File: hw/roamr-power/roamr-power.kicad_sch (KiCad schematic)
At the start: 12 parts, among them J1 Conn_01x02_Socket, J2 Conn_01x02_Socket, J3 Conn_01x02_Socket, P2 USB_C_Plug_USB2.0

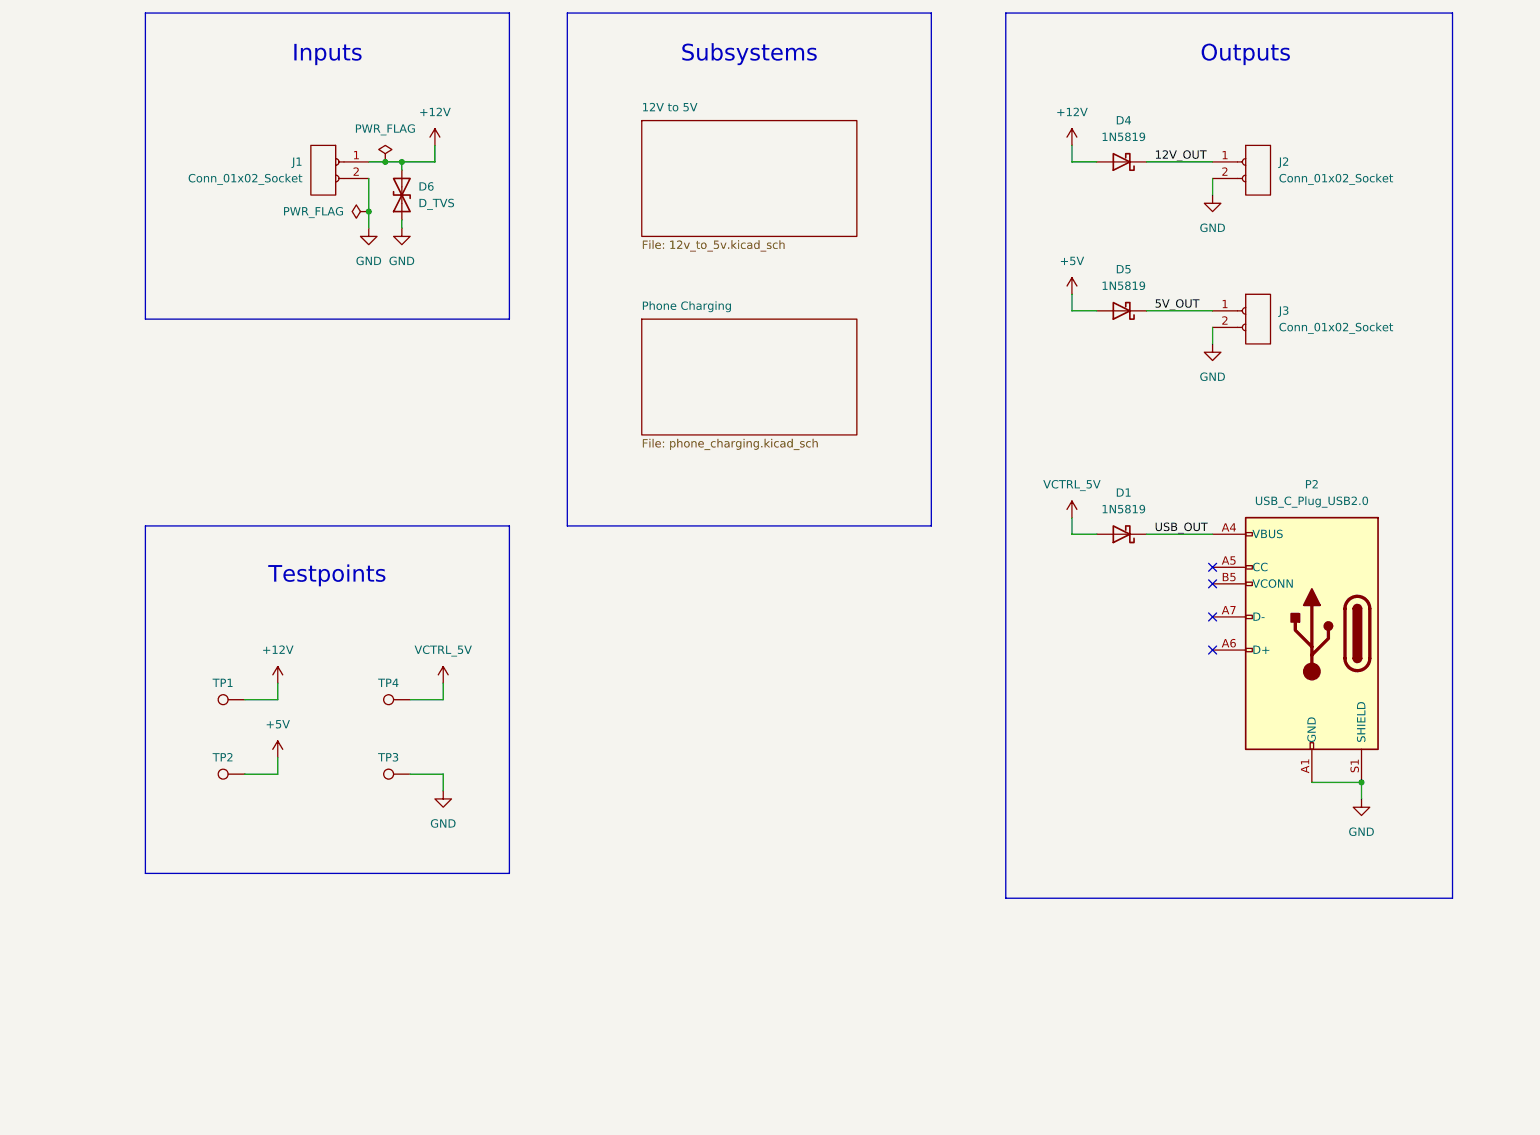
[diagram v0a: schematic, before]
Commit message: pcb schematic and layout updated
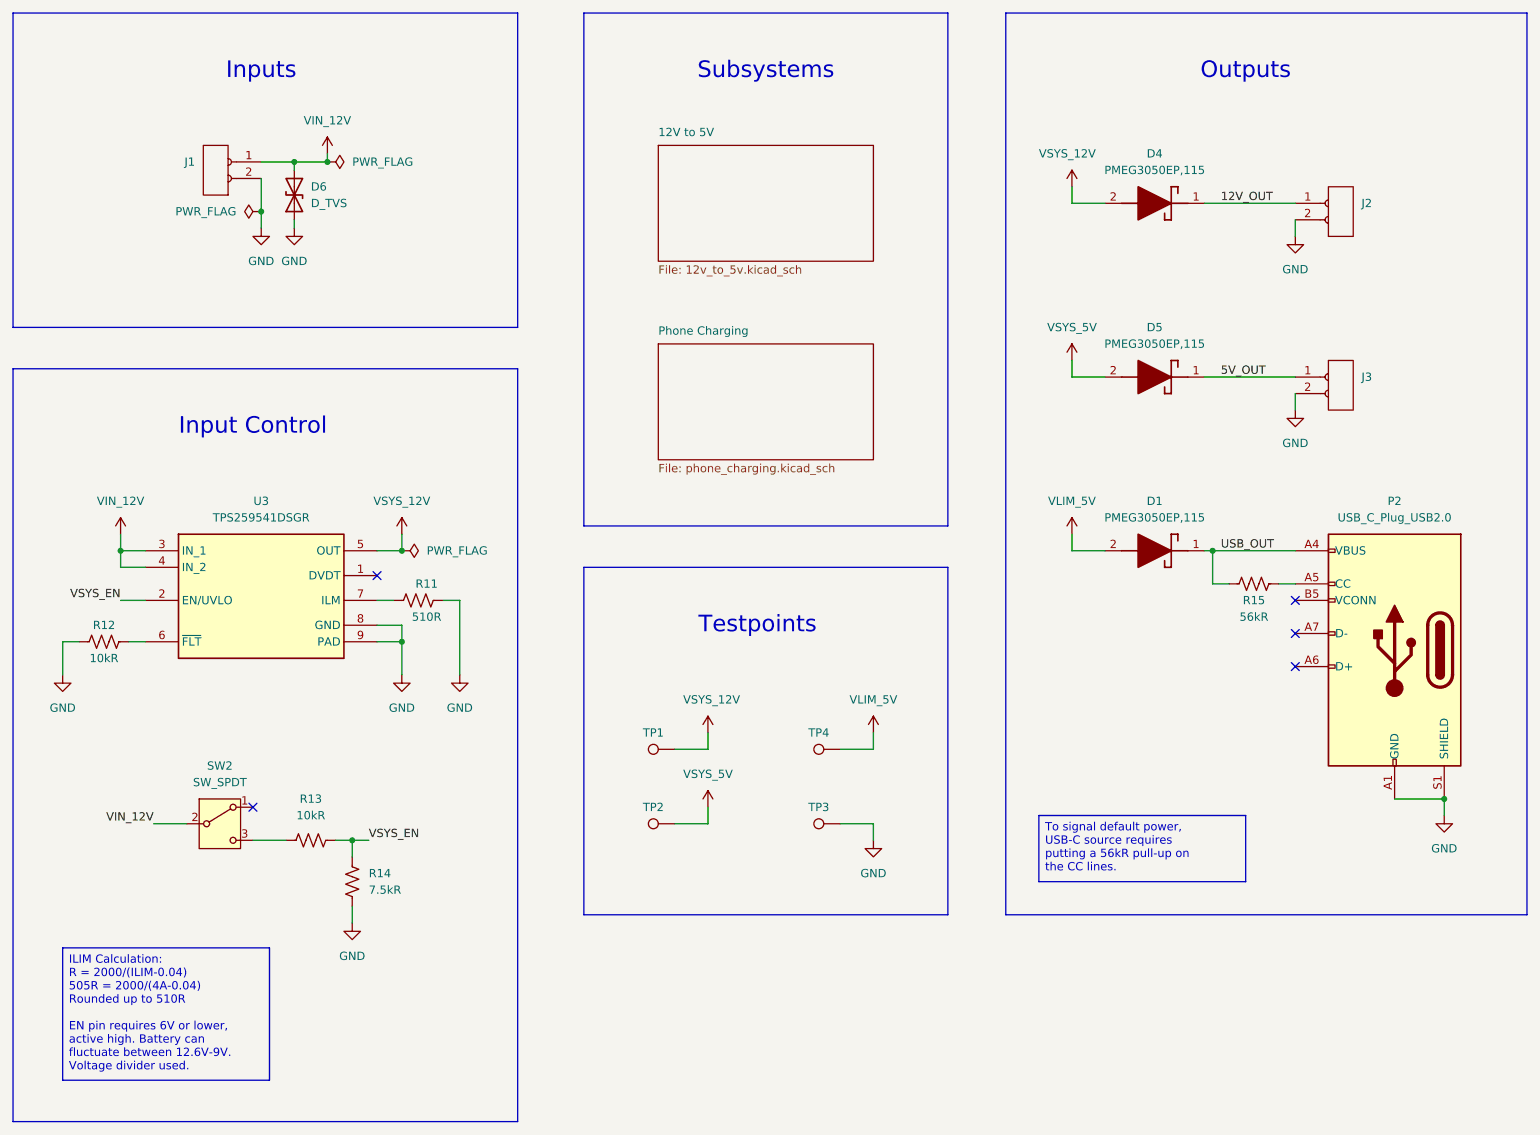
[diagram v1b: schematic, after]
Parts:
- removed D1, D4, D5: 1N5819, Diode_THT:D_DO-41_SOD81_P10.16mm_Horizontal, symbol Diode:1N5819
- added D1, D4, D5: PMEG3050EP,115, PMEG3050EP:PMEG3050EP115, symbol PMEG3050EP_115:PMEG3050EP,115
- added R11: 510R, Resistor_SMD:R_0603_1608Metric, symbol Device:R_US
- added R12, R13: 10kR, Resistor_SMD:R_0603_1608Metric, symbol Device:R_US
- added R14: 7.5kR, Resistor_SMD:R_0603_1608Metric, symbol Device:R_US
- added R15: 56kR, Resistor_SMD:R_0603_1608Metric, symbol Device:R_US
- added SW2: SW_SPDT, OS102011MS2QN1:OS102011MA1QN1, symbol Switch:SW_SPDT
- added U3: TPS259541DSGR, TPS259541DSGR:SON50P200X200X80-9N, symbol TPS259541DSGR:TPS259541DSGR
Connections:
- net 12V_OUT: now also D4.1 (K)
- net 5V_OUT: now also D5.1 (K)
- net GND: now also R11.2, R12.1, R14.2, U3.8 (GND), U3.9 (PAD)
- net USB_OUT: now also D1.1 (K), R15.1
- net at P2.A5 (CC): now also R15.2
- net +12V renamed VIN_12V
- net VIN_12V: now also SW2.2 (B), U3.3 (IN_1), U3.4 (IN_2); no longer TP1.1
- net +5V renamed VSYS_5V
- net VSYS_5V: now also D5.2 (A)
- net VCTRL_5V renamed VLIM_5V
- net VLIM_5V: now also D1.2 (A)
- new net: R12.2, U3.6 (~{FLT})
- new net: R11.1, U3.7 (ILM)
- new net: R13.1, SW2.3 (C)
- new net VSYS_12V: D4.2 (A), TP1.1, U3.5 (OUT)
- new net VSYS_EN: R13.2, R14.1, U3.2 (EN/UVLO)
- no-connect marks 4 -> 5
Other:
- note added: "Input Control"
- moved on the sheet: D6, J1, J2, J3, P2, TP1, TP2, TP3, TP4
